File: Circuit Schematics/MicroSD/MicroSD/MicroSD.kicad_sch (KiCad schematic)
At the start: 46 parts

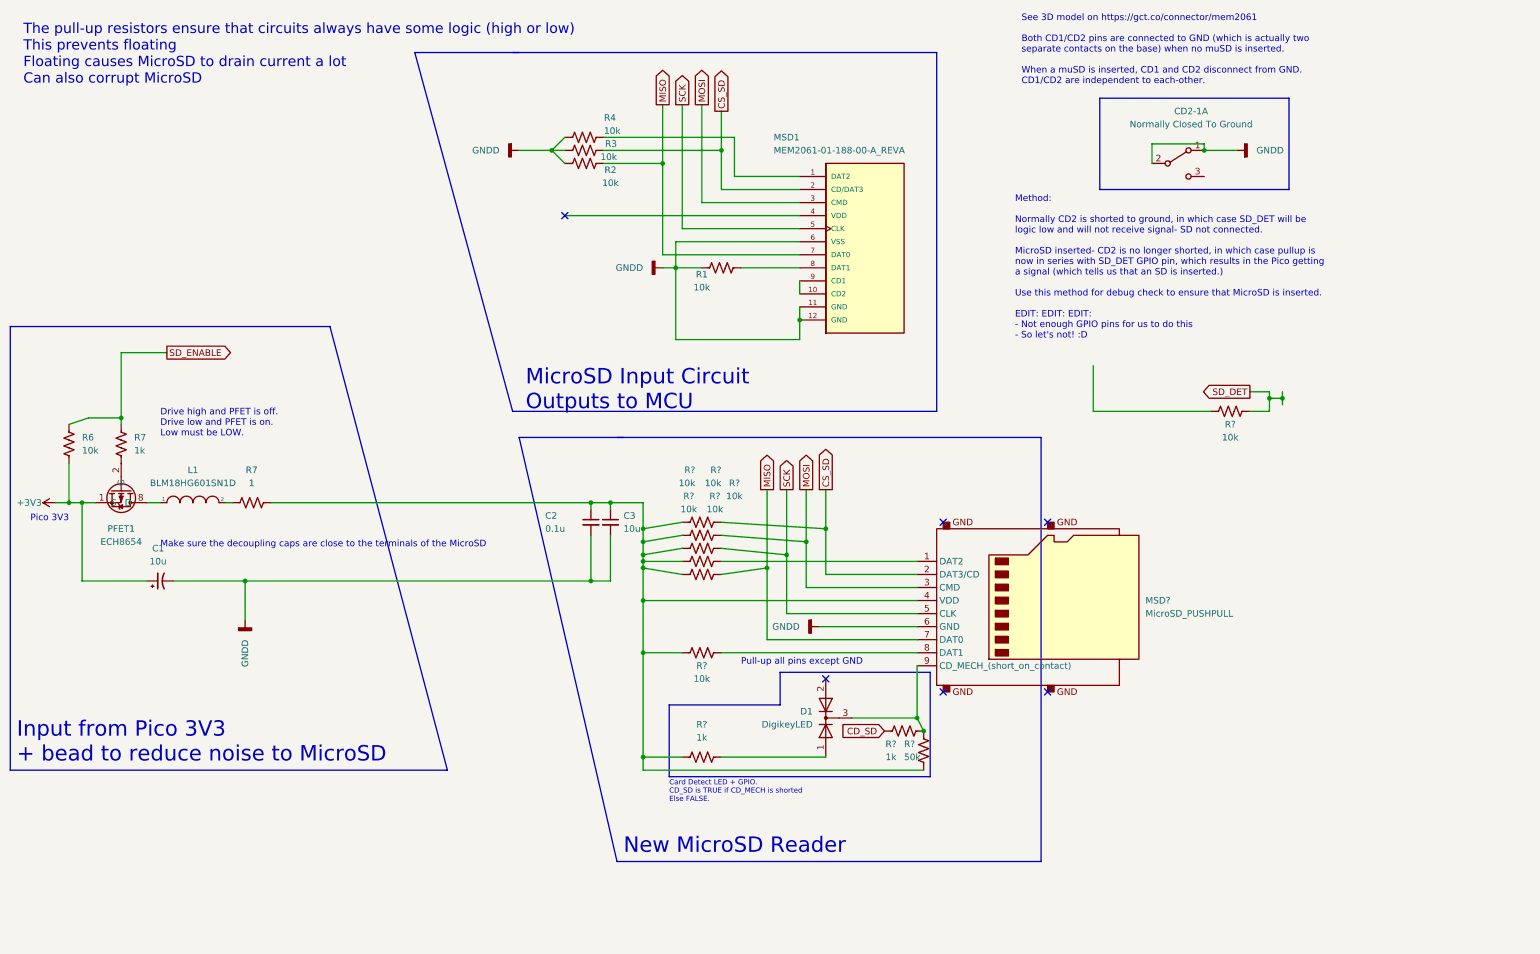
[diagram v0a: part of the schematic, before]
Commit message: Whole boatload of changes
Latest.
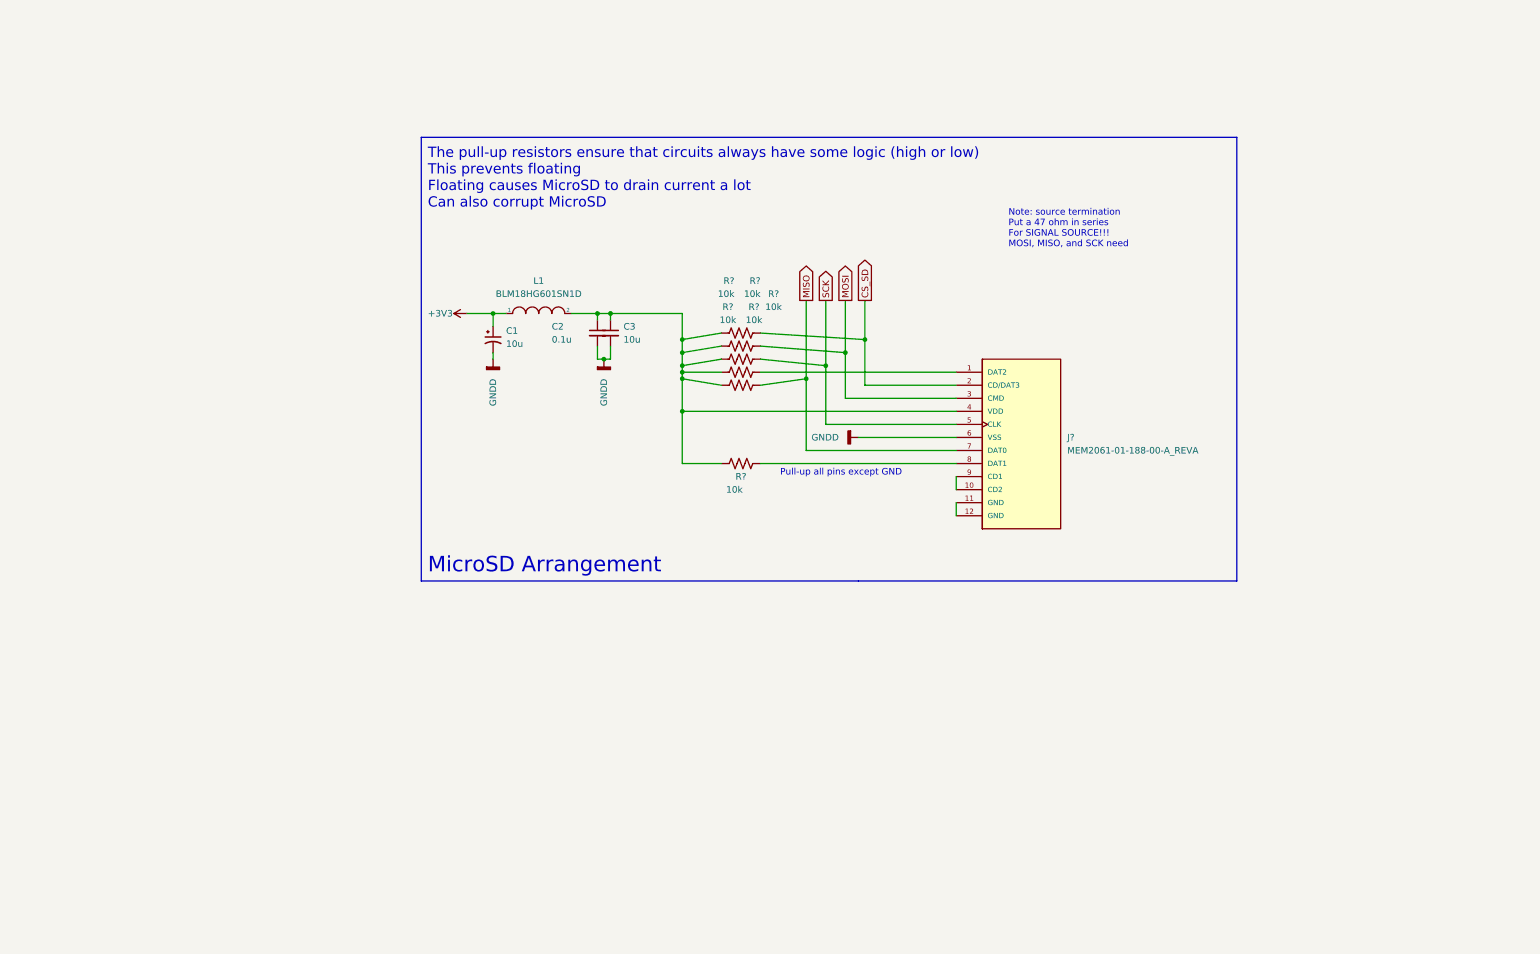
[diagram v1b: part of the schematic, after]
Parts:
- removed CD2-1: Normally Closed To Ground, symbol Switch:SW_DPDT_x2
- removed D1: DigikeyLED, symbol Device:D_Dual_CommonCathode_AAK
- removed MSD1: MEM2061-01-188-00-A_REVA, GCT_MEM2061-01-188-00-A_REVA, symbol MEM2061-01-188-00-A_REVA:MEM2061-01-188-00-A_REVA
- removed MSD?: MicroSD_PUSHPULL, symbol EBAY_MicroSD:MicroSD_PUSHPULL
- removed PFET1: ECH8654, symbol ECH8654-TL-H_PFET:ECH8654
- removed R1, R2, R3, R4, R6, R? (x7): 10k, symbol Device:R_US
- removed R7: 1, symbol Device:R_US
- removed R7, R? (x2): 1k, symbol Device:R_US
- removed R?: 50k, symbol Device:R_US
- added J?: MEM2061-01-188-00-A_REVA, GCT_MEM2061-01-188-00-A_REVA, symbol MEM2061-01-188-00-A_REVA:MEM2061-01-188-00-A_REVA
- added R? (x6): 10k, symbol Device:R_US
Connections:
- net +3V3: now also L1.1
- net CS_SD: now also J?.2 (CD/DAT3), R?.1
- net GNDD: now also J?.6 (VSS)
- net MISO: now also J?.7 (DAT0), R?.2
- net MOSI: now also J?.3 (CMD), R?.2
- net SALEAE_2: now also J?.5 (CLK), R?.1
- net at L1.2: now also C2.1, C3.1, J?.4 (VDD), R?.1, R?.1, R?.1, R?.1, R?.2, R?.2
- new net: J?.1 (DAT2), R?.2
- new net: J?.8 (DAT1), R?.2
- new net: J?.10 (CD2), J?.9 (CD1)
- new net: J?.11 (GND), J?.12 (GND)
- no-connect marks 11 -> 5
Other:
- note added: "MicroSD Arrangement"
- note added: "Note: source termination Put a 47 ohm in series For SIGNAL SOURCE!!! MOSI, MISO, and SCK need"
- note removed: "Method: Normally CD2 is shorted to ground, in which case SD_DET will be logic low and will not receive signal- SD not connected. MicroSD inserted- CD2 is no longer shorted, in which case pullup is now in series with SD_DET GPIO pin, which results in the Pico getting a signal (which tells us that an SD is inserted.) Use this method for debug check to ensure that MicroSD is inserted. EDIT: EDIT: ED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"
- note removed: "MicroSD Input Circuit Outputs to MCU"
- note removed: "See 3D model on https://gct.co/connector/mem2061 Both CD1/CD2 pins are connected to GND (which is actually two separate contacts on the base) when no muSD is inserted. When a muSD is inserted, CD1 and CD2 disconnect from GND. CD1/CD2 are independent to each-other."
- moved on the sheet: C1, C2, C3, L1
